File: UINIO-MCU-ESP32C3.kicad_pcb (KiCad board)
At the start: 2 copper layers, 59.9 x 20.3 mm, 44 parts, among them J1 Conn_01x15_Pin, J2 Conn_01x04_Pin, J3 Conn_01x15_Pin, SW1 复位按键, SW2 下载按键, U1 ME6211C33M5G-N, U2 W25Q128JVSSIQ, U3 ESP32-C3, U4 CH343P, Y1 40MHz

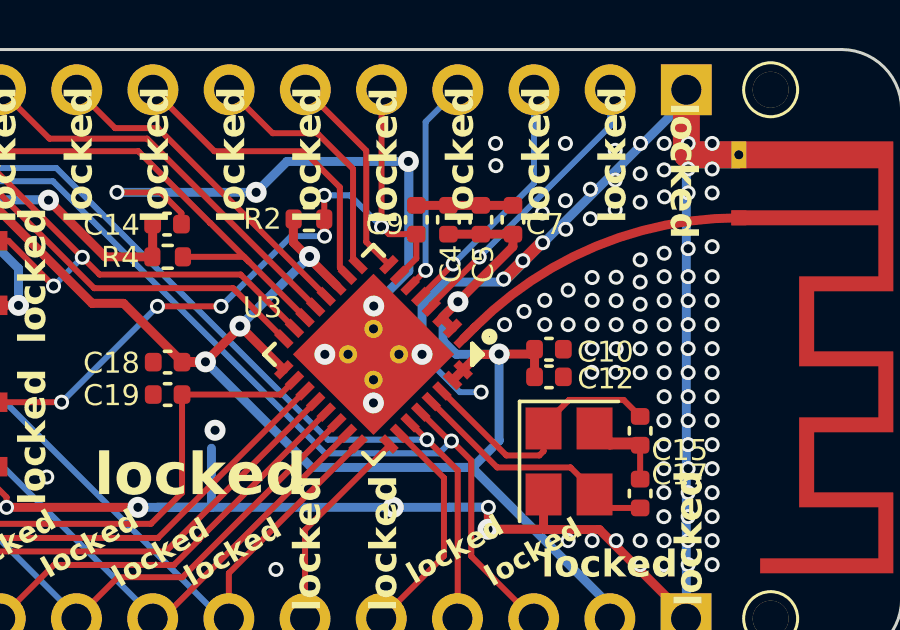
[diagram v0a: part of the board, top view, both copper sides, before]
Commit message: Release UINIO-MCU-ESP32C3 version 3.6.2.
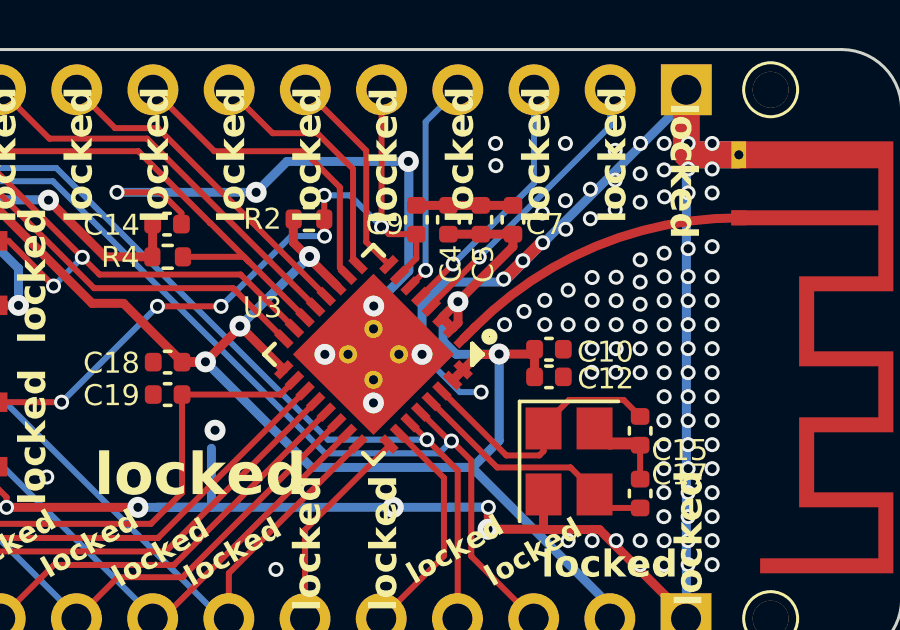
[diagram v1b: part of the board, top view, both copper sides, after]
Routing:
- net /VDD_3.3V: track 145.0 -> 145.9 mm

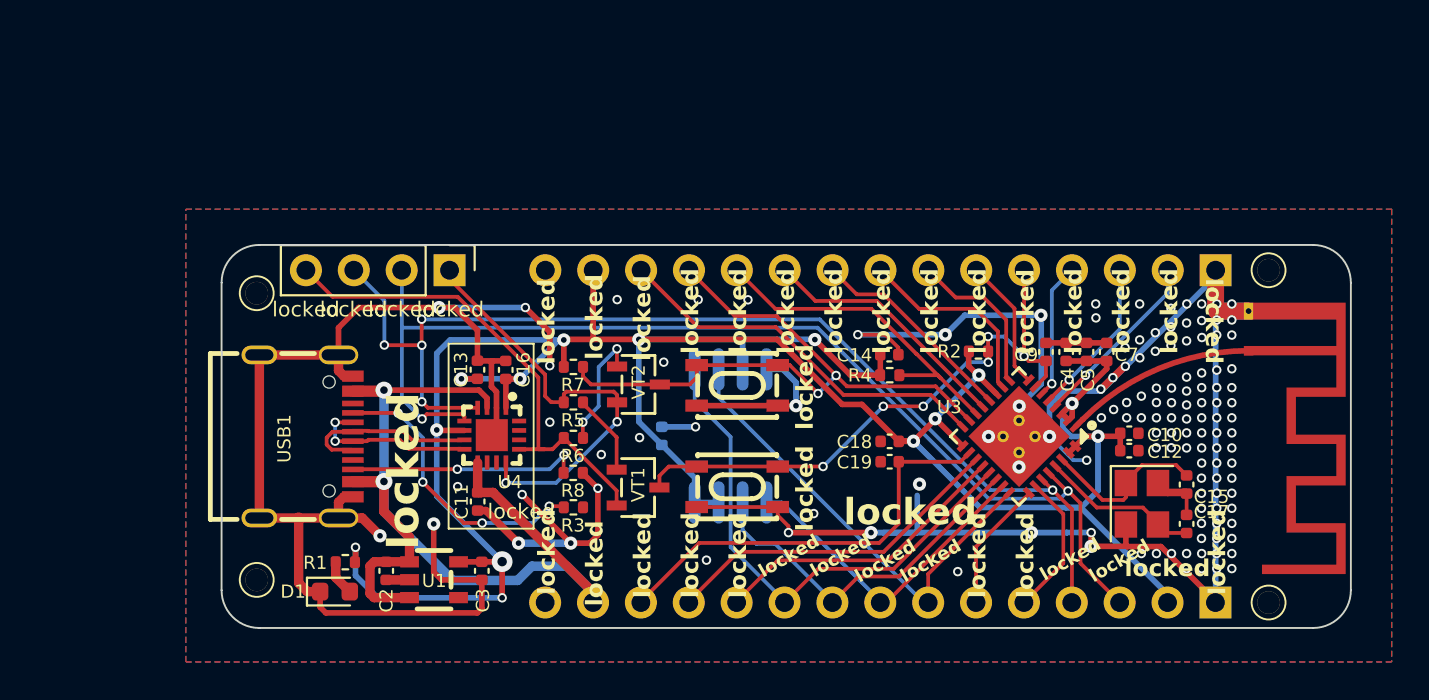
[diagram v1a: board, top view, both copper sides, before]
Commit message: update
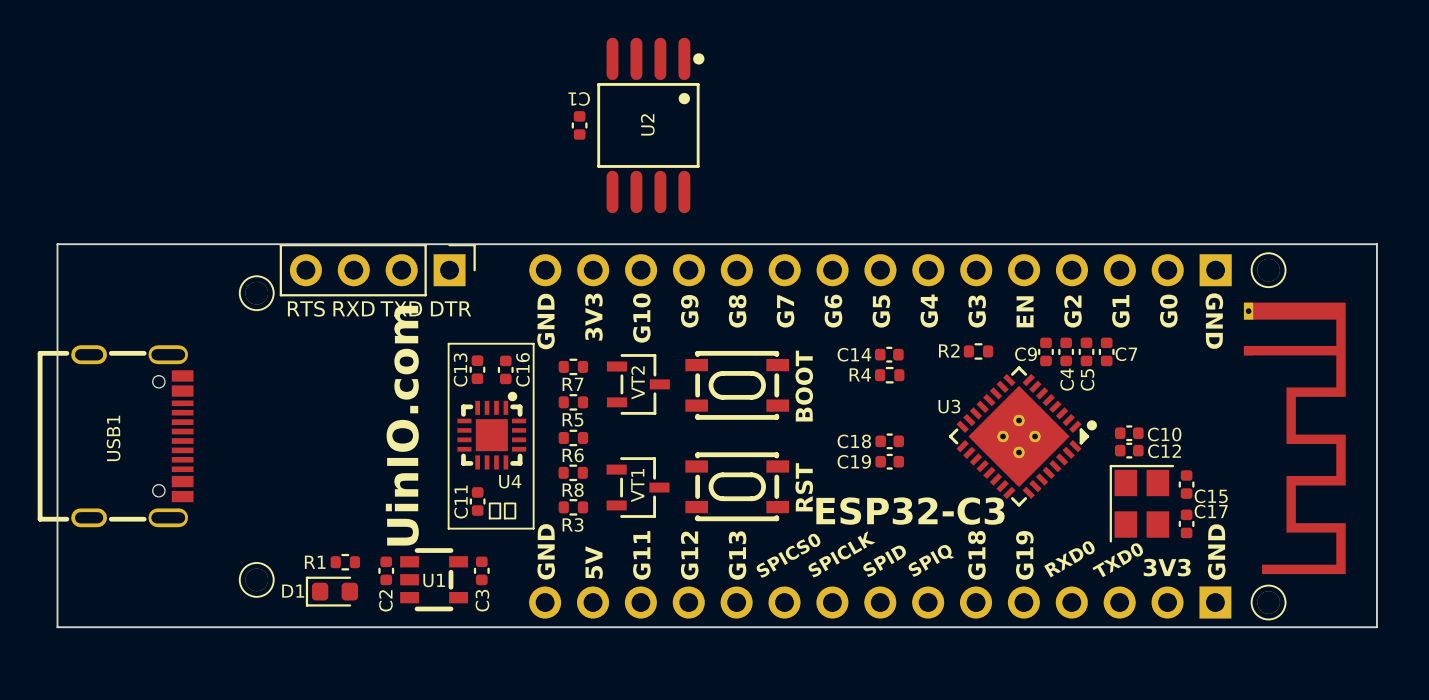
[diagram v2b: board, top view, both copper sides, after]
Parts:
- C1, U2: moved to F.Cu
- moved C1 17.0 mm to (140.0, 86.5)
- moved U2 17.0 mm to (143.7, 86.5), turned to 180 degrees
- moved USB1 9.03 mm to (116.5, 103.0)
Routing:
- net GND: track 204.6 -> 0.00 mm, vias 131 -> 0
- net /VDD_3.3V: track 145.9 -> 0.00 mm, vias 14 -> 0
- net /U0TXD: track 58.7 -> 0.00 mm, vias 2 -> 0
- net /U0RXD: track 58.5 -> 0.00 mm, vias 5 -> 0
- net /VDD_5V: track 50.0 -> 0.00 mm, vias 2 -> 0
- net /GPIO9/BOOT: track 34.1 -> 0.00 mm, vias 2 -> 0
- net /CHIP_EN: track 31.7 -> 0.00 mm, vias 6 -> 0
- net /SPICS0: track 28.0 -> 0.00 mm
- net /RTS: track 26.2 -> 0.00 mm
- net /SPIQ: track 24.2 -> 0.00 mm
- net /VDD_SPI/GPIO11: track 22.6 -> 0.00 mm
- net /DTR: track 22.5 -> 0.00 mm, vias 2 -> 0
- net /GPIO10: track 20.5 -> 0.00 mm
- net /SPICLK: track 19.2 -> 0.00 mm
- net /SPIHD/GPIO12: track 18.4 -> 0.00 mm
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- removed copper zone on B.Cu, net GND
- removed copper zone on F.Cu, net GND
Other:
- board size 59.9 x 20.3 mm -> 70 x 20.3 mm
- board text added: "3V3"
- board text added: "5V"
- board text added: "BOOT"
- board text added: "DTR"
- board text added: "EN"
- board text added: "ESP32-C3"
- board text added: "G0"
- board text added: "G1"
- board text added: "G10"
- board text added: "G11"
- board text added: "G12"
- board text added: "G13"
- board text added: "G18"
- board text added: "G19"
- board text added: "G2"
- board text added: "G3"
- board text added: "G4"
- board text added: "G5"
- board text added: "G6"
- board text added: "G7"
- board text added: "G8"
- board text added: "G9"
- board text added: "GND"
- board text added: "RST"
- board text added: "RTS"
- board text added: "RXD"
- board text added: "RXD0"
- board text added: "SPICLK"
- board text added: "SPICS0"
- board text added: "SPID"
- board text added: "SPIQ"
- board text added: "TXD"
- board text added: "TXD0"
- board text added: "UINIO-MCU-ESP32C3"
- board text added: "UinIO.com"
- board text added: "Version 3.6.2"
- board text added: "可选"
- board text removed: "locked"
